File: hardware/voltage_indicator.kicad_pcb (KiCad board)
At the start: 2 copper layers, 45 x 61 mm, 41 parts, among them J1 HV+, J2 HV-, Q1 TK3P80E,RQ, U1 LT8316EFE, U2 LM211DT

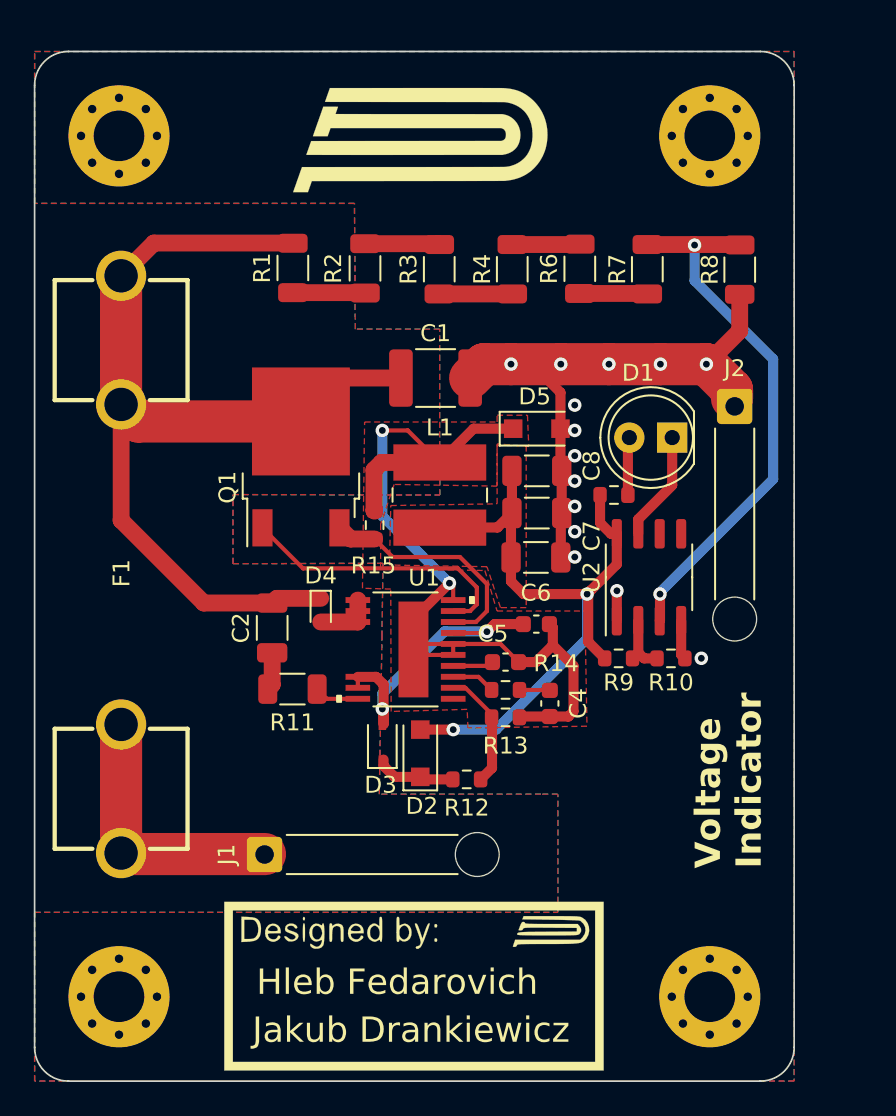
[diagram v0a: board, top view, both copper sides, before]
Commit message: Improve the layout
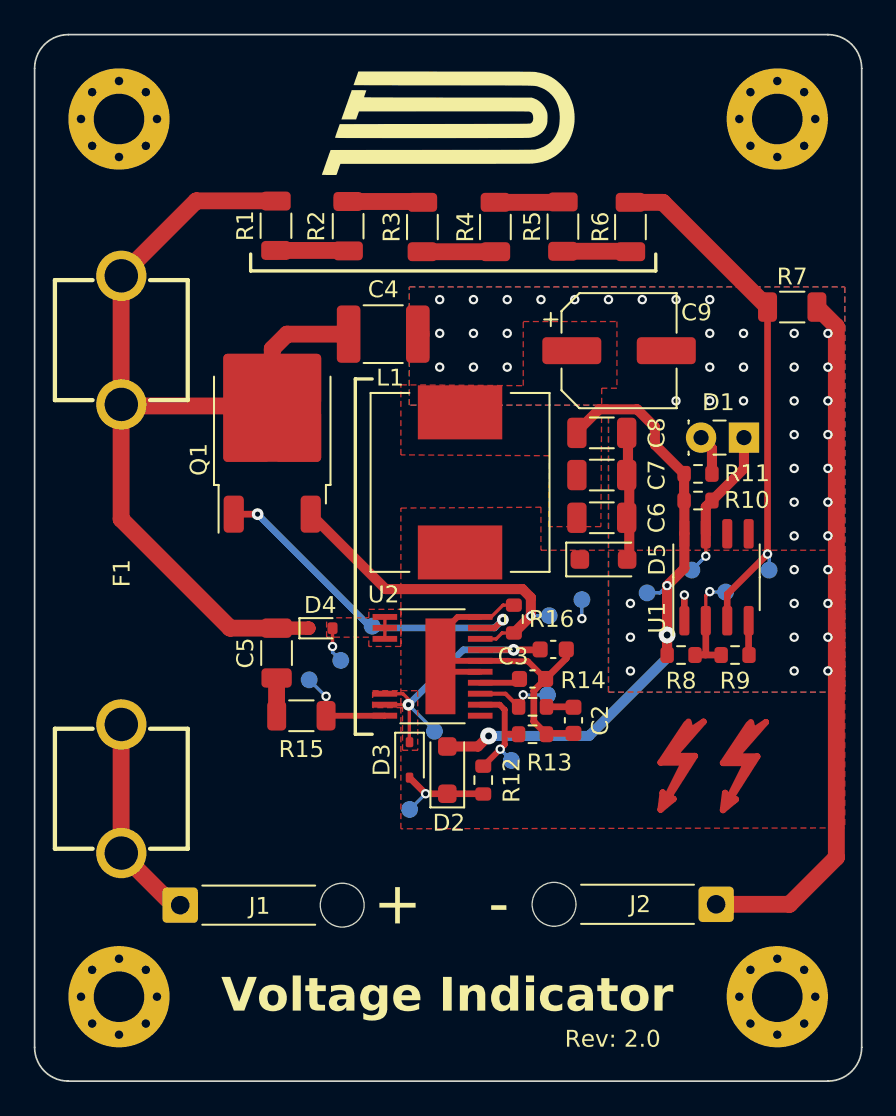
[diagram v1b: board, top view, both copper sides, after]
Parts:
- removed the G*** at (152.4, 75.1)
- added C9: DNP, Capacitor_SMD:CP_Elec_6.3x5.4, F.Cu at (164.6, 87.8)
- added G***: LOGO, Local_Library:putm_15mm, F.Cu at (154.5, 74.3)
- added R10: 1k2, Resistor_SMD:R_0603_1608Metric, F.Cu at (169.3, 96.7)
- added REF**: Symbol_Highvoltage_Type1_CopperTop_Small, Symbol:Symbol_Highvoltage_Type1_CopperTop_Small, F.Cu at (171.2, 113.0)
- added REF**: Symbol_Highvoltage_Type1_CopperTop_Small, Symbol:Symbol_Highvoltage_Type1_CopperTop_Small, F.Cu at (167.5, 112.9)
- added TP1: LM_N, TestPoint:TestPoint_Pad_D1.0mm, B.Cu at (173.5, 100.8)
- added TP10: LT_VIN, TestPoint:TestPoint_Pad_D1.0mm, B.Cu at (148.1, 106.1)
- added TP11: LT_GATE, TestPoint:TestPoint_Pad_D1.0mm, B.Cu at (150.0, 104.1)
- added TP12: LT_SENSE, TestPoint:TestPoint_Pad_D1.0mm, B.Cu at (160.5, 103.5)
- added TP13: LT_VOUT, TestPoint:TestPoint_Pad_D1.0mm, B.Cu at (166.3, 102.1)
- added TP2: LM_P, TestPoint:TestPoint_Pad_D1.0mm, B.Cu at (170.9, 102.1)
- added TP3: LM_OUT, TestPoint:TestPoint_Pad_D1.0mm, B.Cu at (168.9, 100.8)
- added TP4: LT_D3, TestPoint:TestPoint_Pad_D1.0mm, B.Cu at (152.2, 115.0)
- added TP5: LT_VC, TestPoint:TestPoint_Pad_D1.0mm, B.Cu at (160.4, 108.2)
- added TP6: LT_BIAS, TestPoint:TestPoint_Pad_D1.0mm, B.Cu at (153.7, 110.3)
- added TP7: LT_FB, TestPoint:TestPoint_Pad_D1.0mm, B.Cu at (158.2, 112.0)
- added TP8: LT_GND, TestPoint:TestPoint_Pad_D1.0mm, B.Cu at (162.4, 102.5)
- added TP9: LT_DCM, TestPoint:TestPoint_Pad_D1.0mm, B.Cu at (146.3, 107.3)
- C1: renamed from C3; value 10uF -> 10u
- C2: renamed from C4; value 100nF -> 100n
- C3: renamed from C5; value 100nF -> 100n
- C4: renamed from C1; value 0.1uF -> 100n
- C5: renamed from C2; value 10pF -> 10p
- C6, C7, C8: value 47uF -> 47u
- D1: footprint LED_THT:LED_D5.0mm -> LED_THT:LED_Rectangular_W3.9mm_H1.9mm
- D3: value type="D" model="CMDSH2-3" lib="" -> CMDSH2-3
- D4: value D_Zener 10V -> 10V
- F1: value Fuse 600V -> 600V; footprint vindicator:01020071Z-FUSE-CLIP -> Local_Library:FuseClip
- G***: footprint SignatureBox25mm -> Local_Library:SignatureBox25mm; moved to B.Cu
- J1, J2: footprint Connector_Wire:SolderWire-0.5sqmm_1x01_D0.9mm_OD2.1mm_Relief -> Local_Library:SolderWire_Relief
- L1: value 1mH -> 1m; footprint Inductor_SMD:L_Wuerth_WE-PD2-Typ-MS -> Local_Library:WurthElektronikInductor_7687714102
- Q1: value TK3P80E,RQ -> TK3P80ERQ
- R12: value 21.5kR -> 21k5
- R13: value 2.49kR -> 2k49
- R14: value 22.1kR -> 22k1
- R15: renamed from R11; value 10kR -> 10k
- R16: renamed from R15; value 220mR -> 220m
- R9: renamed from R10; value 240 -> 240R
- moved G*** 49.3 mm to (153.2, 76.2), turned to 180 degrees
- moved J2 29.5 mm to (170.4, 120.6), turned to -90 degrees
- moved R16 9.95 mm to (158.4, 103.7)
- moved D5 8.70 mm to (163.7, 100.1)
- moved J1 5.83 mm to (138.6, 120.6)
- moved R11 5.13 mm to (169.3, 95.1)
- moved C6 4.56 mm to (163.6, 97.7)
- moved C7 4.46 mm to (163.6, 95.1)
- moved C8 4.46 mm to (163.6, 92.6)
- moved D1 4.25 mm to (172.0, 92.9)
- moved REF** 4.12 mm to (174.0, 74.0)
- moved C4 4.05 mm to (150.7, 86.8)
- moved REF** 4.00 mm to (174.0, 126.0)
- moved U1 4.00 mm to (170.4, 101.2)
- moved R7 3.82 mm to (174.9, 85.2), turned to 180 degrees
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- renumbered R5 to R11, R6 to R5, R7 to R6, R8 to R7, R9 to R8, U2 to U1, U1 to U2
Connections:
- D3 pad 1: Net-(D2-K) -> Net-(D3-K)
- D3 pad 2: Net-(D3-K) -> Net-(D2-K)
- F1 pad 1: +VDC -> VCC
- F1 pad 2: Net-(F1-Pad2) -> Net-(J1-Pin_1)
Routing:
- net +VDC: track 57.5 -> 0.00 mm
- net VCC: track 0.00 -> 56.6 mm
- net Net-(D5-K): track 57.3 -> 27.0 mm, vias 2 -> 1
- net Net-(F1-Pad2): track 16.2 -> 0.00 mm
- net Net-(J1-Pin_1): track 0.00 -> 12.4 mm
- net GND: track 42.0 -> 52.8 mm, vias 14 -> 48
- net Net-(Q1-S): track 14.0 -> 20.8 mm, vias 0 -> 1
- net +12V: track 42.5 -> 38.2 mm, vias 2 -> 3
- net Net-(Q1-G): track 16.7 -> 20.5 mm, vias 0 -> 2
- net Net-(U2-DCM): track 2.65 -> 6.04 mm, vias 0 -> 1
- net Net-(U1-+): track 3.62 -> 6.36 mm, vias 0 -> 1
- net Net-(D1-K): track 6.53 -> 9.13 mm, vias 0 -> 1
- net Net-(U2-VC): track 2.60 -> 4.86 mm, vias 0 -> 1
- net Net-(D2-K): track 4.81 -> 6.11 mm, vias 0 -> 1
- net Net-(U1--): track 32.5 -> 31.3 mm, vias 2 -> 1
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- added copper zone on F.Cu, net Net-(D3-K)
- added copper zone on F.Cu, net Net-(D4-A)
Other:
- board size 45 x 61 mm -> 49 x 62 mm
- board text added: "+"
- board text added: "-"
- board text added: "Hleb Fedarovich"
- board text added: "Jakub Drankiewicz"
- board text added: "Rev: 2.0"
